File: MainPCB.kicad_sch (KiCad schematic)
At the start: 74 parts, among them IC1 VNH7070ASTR, IC2 VNH7070ASTR, IC3 VNH7070ASTR, IC4 VNH7070ASTR, J1 Conn_01x06, J10 Conn_01x02, J11 Conn_01x03, J2 RaspberryPi, J3 Conn_01x12, J4 Conn_01x02, J5 Screw_Terminal_01x02, J6 Conn_01x03, J8 Conn_01x02, J9 Conn_01x02, M1 Motor_DC, M2 Motor_DC, M3 Motor_DC, M4 Motor_DC, SW1 SW_DPST_x2, SW2 SW_SPDT, SW3 SW_SPDT, SW4 SW_SPDT, SW5 SW_SPDT, SW6 SW_DPST_x2, U1 V_Regulator3.3v, U10 N channel, U12 Teensy4.1, U2 V_Regulator5v, U3 BoostConverter, U6 N channel, U7 4554

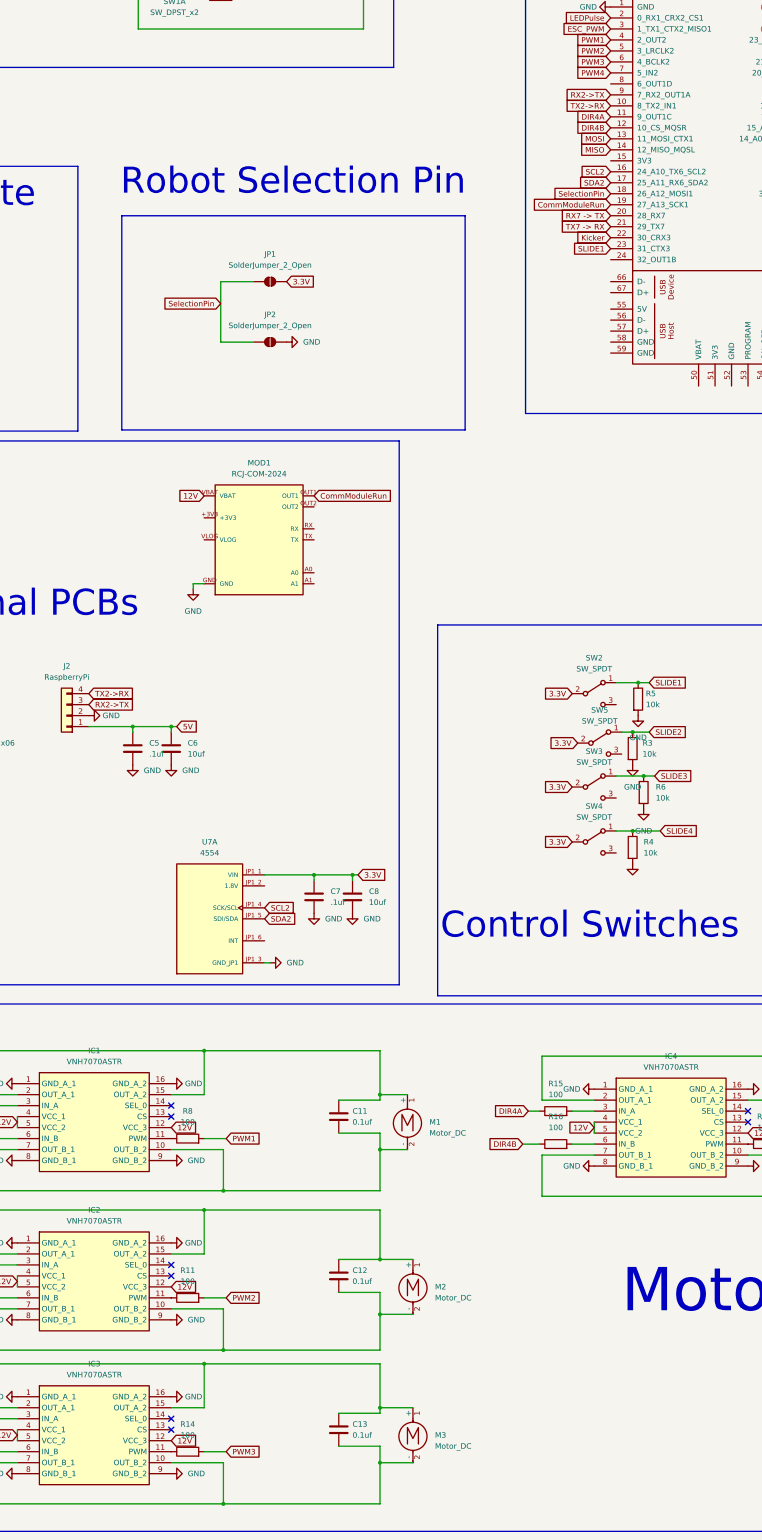
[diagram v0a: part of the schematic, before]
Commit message: Placement Done
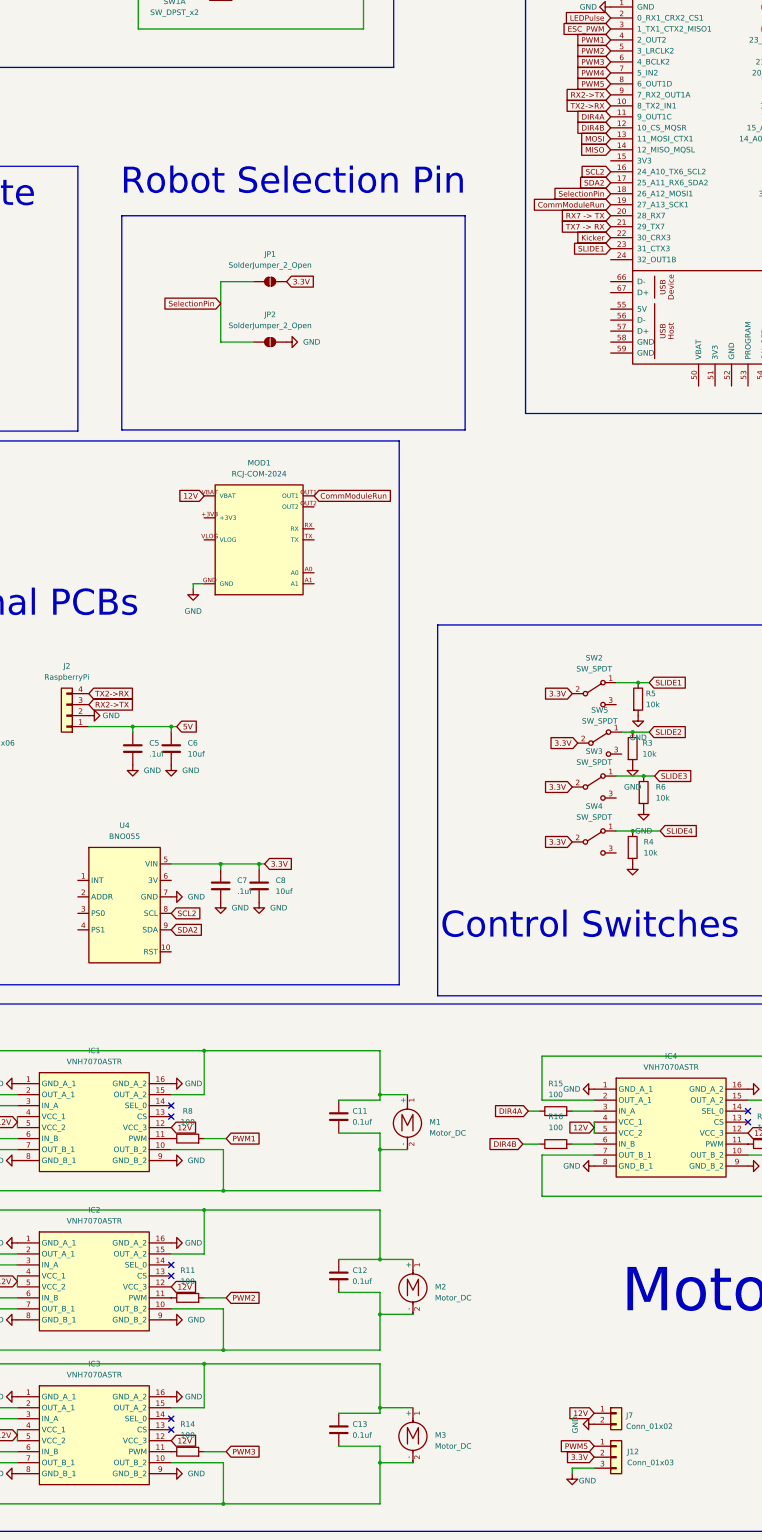
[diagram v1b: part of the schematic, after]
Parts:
- removed U7: 4554, 4554:MODULE_4554, symbol 4554:4554
- added J12: Conn_01x03, Connector_JST:JST_XH_B3B-XH-A_1x03_P2.50mm_Vertical, symbol Connector_Generic:Conn_01x03
- added J7: Conn_01x02, Connector_JST:JST_XH_B2B-XH-A_1x02_P2.50mm_Vertical, symbol Connector_Generic:Conn_01x02
- added U4: BNO055, BNO055:BNO055, symbol AdafruitBNO055:BNO055
- J10, J8, J9: footprint Connector_PinHeader_2.54mm:PinHeader_1x02_P2.54mm_Vertical -> Connector_JST:JST_XH_B2B-XH-A_1x02_P2.50mm_Vertical
- J11: footprint Connector_PinHeader_2.54mm:PinHeader_1x03_P2.54mm_Vertical -> Connector_JST:JST_XH_B3B-XH-A_1x03_P2.50mm_Vertical
- JP1, JP2: footprint (none) -> Jumper:SolderJumper-2_P1.3mm_Open_RoundedPad1.0x1.5mm
- M1, M2, M3, M4: footprint Connector_JST:JST_XH_B2B-XH-AM_1x02_P2.50mm_Vertical -> Connector_JST:JST_XH_B2B-XH-A_1x02_P2.50mm_Vertical
- MOD1: footprint RCJ-COM-2024:RCJ-COM-2024 -> RCJ-COM-MOD:RCJ-COM-2024
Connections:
- net 12V: now also J7.1 (Pin_1)
- net 3.3V: now also J12.2 (Pin_2), U4.5 (VIN)
- net GND: now also J12.3 (Pin_3), J7.2 (Pin_2), U4.7 (GND)
- net SCL2: now also U4.8 (SCL)
- net SDA2: now also U4.9 (SDA)
- net PWM5: now reaches U12.8 (6_OUT1D)
- net PWM5: now also J12.1 (Pin_1)
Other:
- moved on the sheet: C7, C8
